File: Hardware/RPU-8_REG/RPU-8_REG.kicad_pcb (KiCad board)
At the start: 4 copper layers, 139.7 x 55.9 mm, 30 parts, among them J1 DATA_BUS, J2 ADDR_BUS, J3 CTRL_BUS, J4 Conn_01x03_Female, J5 REG_CTRL, J6 INST_BITS, U1 74HC245, U2 74HC245, U3 74HC377, U4 74HC377, U5 74HC138, U6 74HC138

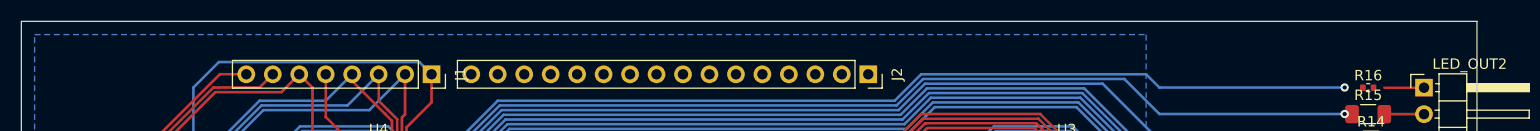
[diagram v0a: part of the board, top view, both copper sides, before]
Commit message: add .readthedocs.yaml
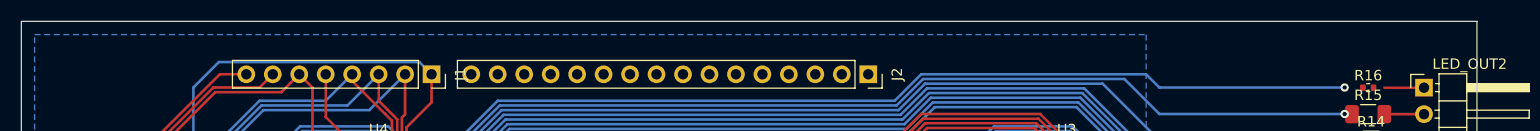
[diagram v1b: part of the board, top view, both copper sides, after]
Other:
- outline, holes or cut-outs redrawn
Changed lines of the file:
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@@
     )
   )
-  (gr_line (start 116.84 78.74) (end 254 78.74) (layer "Edge.Cuts") (width 0.1))
-  (gr_line (start 114.3 134.62) (end 114.3 78.74) (layer "Edge.Cuts") (width 0.1))
-  (gr_line (start 254 134.62) (end 114.3 134.62) (layer "Edge.Cuts") (width 0.1))
-  (gr_line (start 254 78.74) (end 254 134.62) (layer "Edge.Cuts") (width 0.1))
-  (gr_line (start 114.3 78.74) (end 116.84 78.74) (layer "Edge.Cuts") (width 0.1))
+  (gr_rect (start 114.3 78.74) (end 254 134.62) (layer "Edge.Cuts") (width 0.1) (fill none))
   (segment (start 153.67 83.82) (end 153.67 86.505) (width 0.25) (layer "F.Cu") (net 1))
   (segment (start 153.67 86.505) (end 151.275 88.9) (width 0.25) (layer "F.Cu") (net 1))
